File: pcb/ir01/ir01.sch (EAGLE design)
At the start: 9 parts

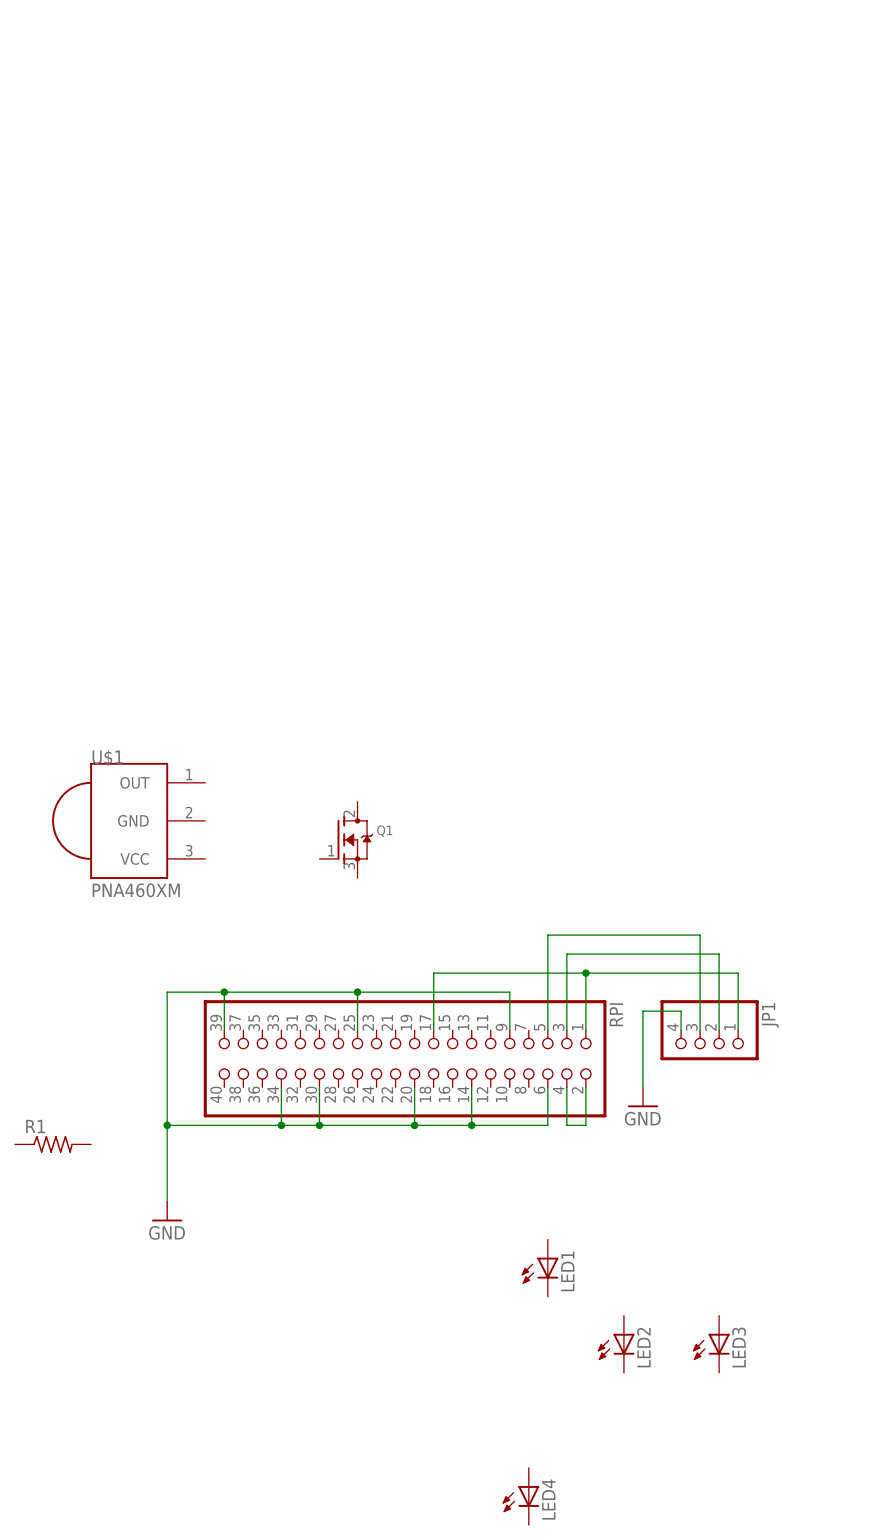
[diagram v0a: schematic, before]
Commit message: update
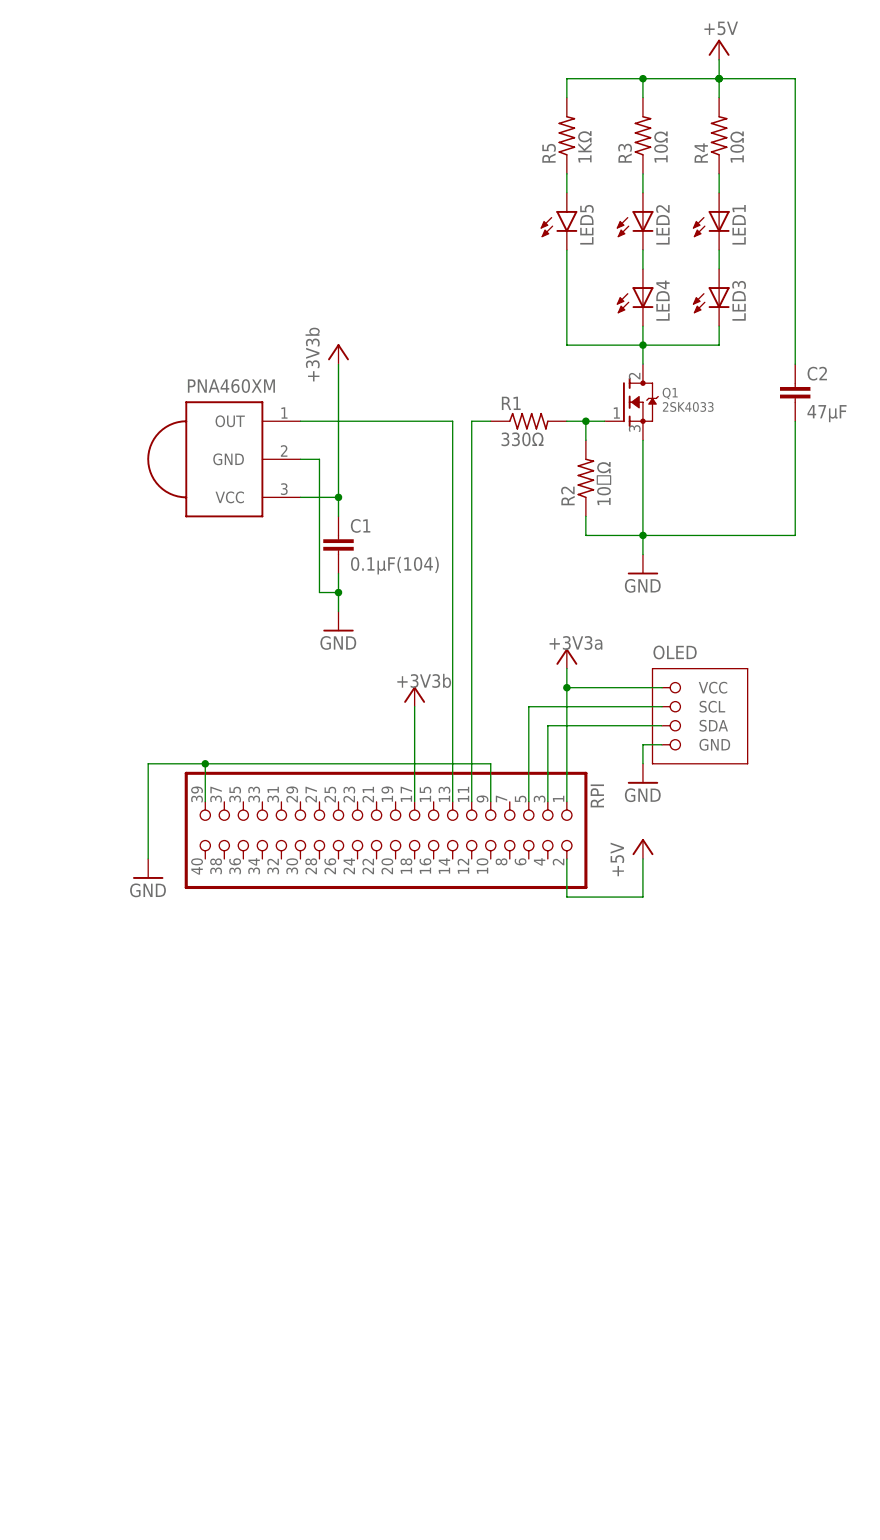
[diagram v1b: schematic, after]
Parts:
- removed JP1: (no value), pinhead:PINHD-1X4
- added C1: 0.1μF(104), rcl:C-EU025-024X044
- added C2: 47μF, rcl:C-EU025-024X044
- added LED5: (no value), led:LED3MM
- added OLED: OLED-SSD1306-0.96, ytani1:OLED-SSD1306-0.96
- added R2: 10ｋΩ, rcl:R-US_0204/5
- added R3, R4: 10Ω, rcl:R-US_0204/5
- added R5: 1KΩ, rcl:R-US_0204/5
- Q1: value (none) -> 2SK4033
- R1: value (none) -> 330Ω
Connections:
- removed net N$1: JP1.1, RPI.1, RPI.17
- removed net N$2: JP1.2, RPI.3
- removed net N$3: JP1.3, RPI.5
- removed net N$6: RPI.2, RPI.4
- new net +3V3A: OLED.VCC, RPI.1
- new net +3V3B: C1.1, RPI.17, U$1.VCC
- new net +5V: C2.1, R3.2, R4.2, R5.2, RPI.2
- new net IRIN: RPI.13, U$1.OUT
- new net IROUT: R1.1, RPI.11
- new net IROUT2: Q1.G, R1.2, R2.2
- new net LEDIN0: LED5.A, R5.1
- new net LEDIN1: LED2.A, R3.1
- new net LEDIN2: LED1.A, R4.1
- new net N$5: LED2.C, LED4.A
- new net N$7: LED1.C, LED3.A
- new net Q1IN: LED3.C, LED4.C, LED5.C, Q1.D
- new net SCL: OLED.SCL, RPI.5
- new net SDA: OLED.SDA, RPI.3
- net GND: now also C1.2, C2.2, OLED.GND, Q1.S, R2.1, U$1.GND; no longer JP1.4, RPI.14, RPI.20, RPI.25, RPI.30, RPI.34, RPI.6
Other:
- moved on the sheet: LED1, LED2, LED3, LED4, Q1, R1, RPI
